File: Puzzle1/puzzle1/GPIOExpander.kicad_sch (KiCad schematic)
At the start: 4 parts, among them J2 Conn_01x16_Pin, U2 PCA9555D

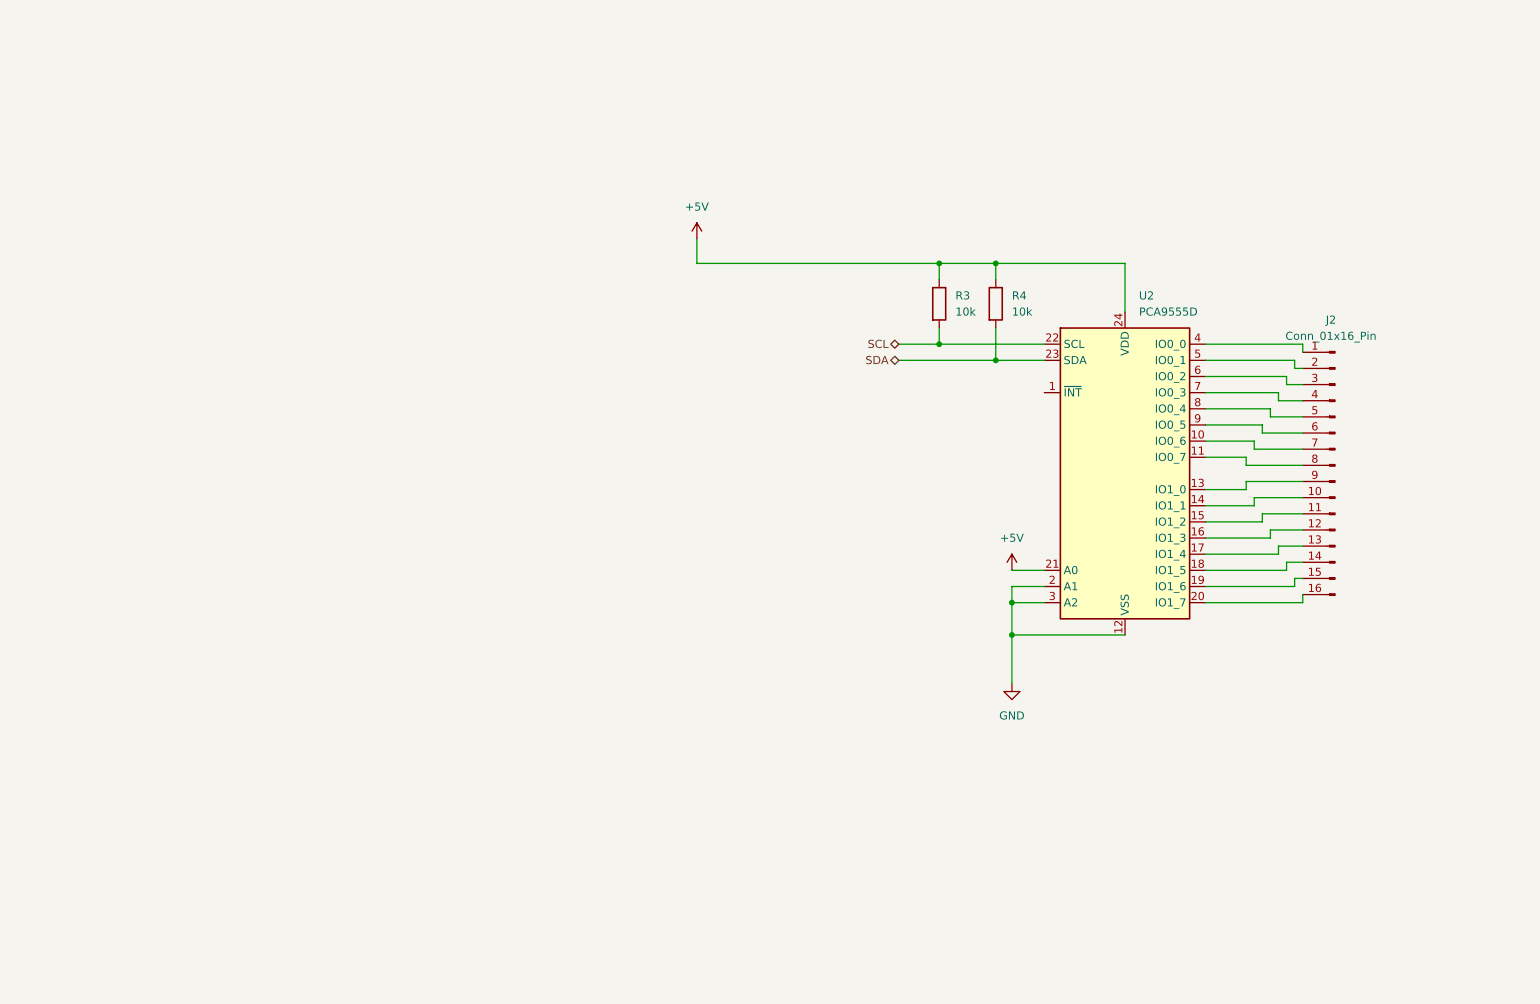
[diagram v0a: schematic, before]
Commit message: update
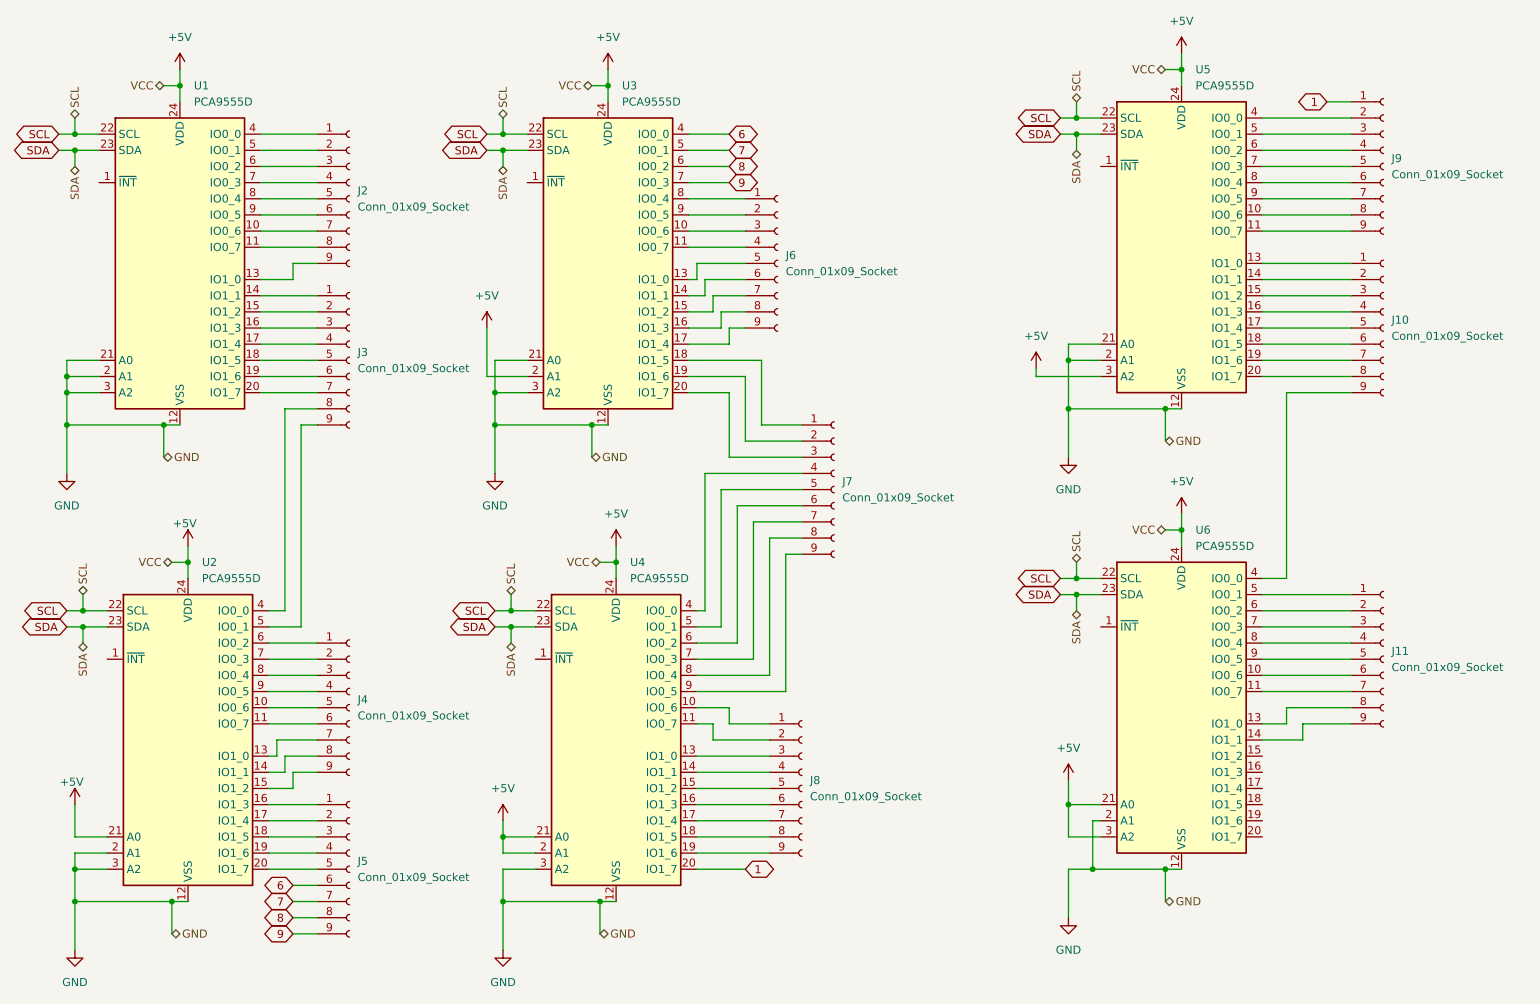
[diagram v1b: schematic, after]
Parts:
- removed J2: Conn_01x16_Pin, Connector_PinSocket_2.54mm:PinSocket_2x09_P2.54mm_Vertical, symbol Connector:Conn_01x16_Pin
- removed R3, R4: 10k, Resistor_SMD:R_0805_2012Metric, symbol Device:R
- added J10, J11, J2, J3, J4, J5, J6, J7, J8, J9: Conn_01x09_Socket, Connector_JST:JST_XH_B9B-XH-A_1x09_P2.50mm_Vertical, symbol Connector:Conn_01x09_Socket
- added U2, U3, U4, U5, U6: PCA9555D, Package_SO:SOIC-24W_7.5x15.4mm_P1.27mm, symbol Interface_Expansion:PCA9555D
- renumbered U2 to U1
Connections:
- net +5V: now also U2.21 (A0), U2.24 (VDD), U3.2 (A1), U3.24 (VDD), U4.2 (A1), U4.21 (A0), U4.24 (VDD), U5.24 (VDD), U5.3 (A2), U6.21 (A0), U6.24 (VDD), U6.3 (A2); no longer U1.21 (A0)
- net GND: now also U1.21 (A0), U2.12 (VSS), U2.2 (A1), U2.3 (A2), U3.12 (VSS), U3.21 (A0), U3.3 (A2), U4.12 (VSS), U4.3 (A2), U5.12 (VSS), U5.2 (A1), U5.21 (A0), U6.12 (VSS), U6.2 (A1)
- net SCL: now also U2.22 (SCL), U3.22 (SCL), U4.22 (SCL), U5.22 (SCL), U6.22 (SCL)
- net SDA: now also U2.23 (SDA), U3.23 (SDA), U4.23 (SDA), U5.23 (SDA), U6.23 (SDA)
- net at U1.4 (IO0_0): now also J2.1 (Pin_1)
- net at U1.14 (IO1_1): now also J3.1 (Pin_1)
- net at U1.15 (IO1_2): now also J3.2 (Pin_2)
- net at U1.16 (IO1_3): now also J3.3 (Pin_3)
- net at U1.17 (IO1_4): now also J3.4 (Pin_4)
- net at U1.18 (IO1_5): now also J3.5 (Pin_5)
- net at U1.19 (IO1_6): now also J3.6 (Pin_6)
- net at U1.20 (IO1_7): now also J3.7 (Pin_7)
- net at U1.5 (IO0_1): now also J2.2 (Pin_2)
- net at U1.6 (IO0_2): now also J2.3 (Pin_3)
- net at U1.7 (IO0_3): now also J2.4 (Pin_4)
- net at U1.8 (IO0_4): now also J2.5 (Pin_5)
- net at U1.9 (IO0_5): now also J2.6 (Pin_6)
- net at U1.10 (IO0_6): now also J2.7 (Pin_7)
- net at U1.11 (IO0_7): now also J2.8 (Pin_8)
- net at U1.13 (IO1_0): now also J2.9 (Pin_9)
- new net: J5.1 (Pin_1), U2.16 (IO1_3)
- new net: J5.2 (Pin_2), U2.17 (IO1_4)
- new net: J5.3 (Pin_3), U2.18 (IO1_5)
- new net: J5.4 (Pin_4), U2.19 (IO1_6)
- new net: J5.5 (Pin_5), U2.20 (IO1_7)
- new net: J10.1 (Pin_1), U5.13 (IO1_0)
- new net: J10.2 (Pin_2), U5.14 (IO1_1)
- new net: J10.3 (Pin_3), U5.15 (IO1_2)
- new net: J10.4 (Pin_4), U5.16 (IO1_3)
- new net: J10.5 (Pin_5), U5.17 (IO1_4)
- new net: J10.6 (Pin_6), U5.18 (IO1_5)
- new net: J10.7 (Pin_7), U5.19 (IO1_6)
- new net: J10.8 (Pin_8), U5.20 (IO1_7)
- new net: J10.9 (Pin_9), U6.4 (IO0_0)
- new net: J6.3 (Pin_3), U3.10 (IO0_6)
- new net: J6.4 (Pin_4), U3.11 (IO0_7)
- new net: J6.5 (Pin_5), U3.13 (IO1_0)
- new net: J6.6 (Pin_6), U3.14 (IO1_1)
- new net: J6.7 (Pin_7), U3.15 (IO1_2)
- new net: J6.8 (Pin_8), U3.16 (IO1_3)
- new net: J6.9 (Pin_9), U3.17 (IO1_4)
- new net: J7.1 (Pin_1), U3.18 (IO1_5)
- new net: J7.2 (Pin_2), U3.19 (IO1_6)
- new net: J7.3 (Pin_3), U3.20 (IO1_7)
- new net: J6.1 (Pin_1), U3.8 (IO0_4)
- new net: J6.2 (Pin_2), U3.9 (IO0_5)
- new net: J11.1 (Pin_1), U6.5 (IO0_1)
- new net: J11.2 (Pin_2), U6.6 (IO0_2)
- new net: J11.3 (Pin_3), U6.7 (IO0_3)
- new net: J11.4 (Pin_4), U6.8 (IO0_4)
- new net: J11.5 (Pin_5), U6.9 (IO0_5)
- new net: J11.6 (Pin_6), U6.10 (IO0_6)
- new net: J11.7 (Pin_7), U6.11 (IO0_7)
- new net: J11.8 (Pin_8), U6.13 (IO1_0)
- new net: J11.9 (Pin_9), U6.14 (IO1_1)
- new net: J8.1 (Pin_1), U4.10 (IO0_6)
- new net: J8.2 (Pin_2), U4.11 (IO0_7)
- new net: J8.3 (Pin_3), U4.13 (IO1_0)
- new net: J8.4 (Pin_4), U4.14 (IO1_1)
- new net: J8.5 (Pin_5), U4.15 (IO1_2)
- new net: J8.6 (Pin_6), U4.16 (IO1_3)
- new net: J8.7 (Pin_7), U4.17 (IO1_4)
- new net: J8.8 (Pin_8), U4.18 (IO1_5)
- new net: J8.9 (Pin_9), U4.19 (IO1_6)
- new net: J9.8 (Pin_8), U5.10 (IO0_6)
- new net: J9.9 (Pin_9), U5.11 (IO0_7)
- new net: J9.2 (Pin_2), U5.4 (IO0_0)
- new net: J9.3 (Pin_3), U5.5 (IO0_1)
- new net: J9.4 (Pin_4), U5.6 (IO0_2)
- new net: J9.5 (Pin_5), U5.7 (IO0_3)
- new net: J9.6 (Pin_6), U5.8 (IO0_4)
- new net: J9.7 (Pin_7), U5.9 (IO0_5)
- new net: J4.1 (Pin_1), U2.6 (IO0_2)
- new net: J4.2 (Pin_2), U2.7 (IO0_3)
- new net: J4.3 (Pin_3), U2.8 (IO0_4)
- new net: J4.4 (Pin_4), U2.9 (IO0_5)
- new net: J4.5 (Pin_5), U2.10 (IO0_6)
- new net: J4.6 (Pin_6), U2.11 (IO0_7)
- new net: J4.7 (Pin_7), U2.13 (IO1_0)
- new net: J4.8 (Pin_8), U2.14 (IO1_1)
- new net: J4.9 (Pin_9), U2.15 (IO1_2)
- new net: J7.4 (Pin_4), U4.4 (IO0_0)
- new net: J7.5 (Pin_5), U4.5 (IO0_1)
- new net: J7.6 (Pin_6), U4.6 (IO0_2)
- new net: J7.7 (Pin_7), U4.7 (IO0_3)
- new net: J7.8 (Pin_8), U4.8 (IO0_4)
- new net: J7.9 (Pin_9), U4.9 (IO0_5)
- new net: J3.8 (Pin_8), U2.4 (IO0_0)
- new net: J3.9 (Pin_9), U2.5 (IO0_1)
- new net 1: J9.1 (Pin_1), U4.20 (IO1_7)
- new net 6: J5.6 (Pin_6), U3.4 (IO0_0)
- new net 7: J5.7 (Pin_7), U3.5 (IO0_1)
- new net 8: J5.8 (Pin_8), U3.6 (IO0_2)
- new net 9: J5.9 (Pin_9), U3.7 (IO0_3)
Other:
- moved on the sheet: U1

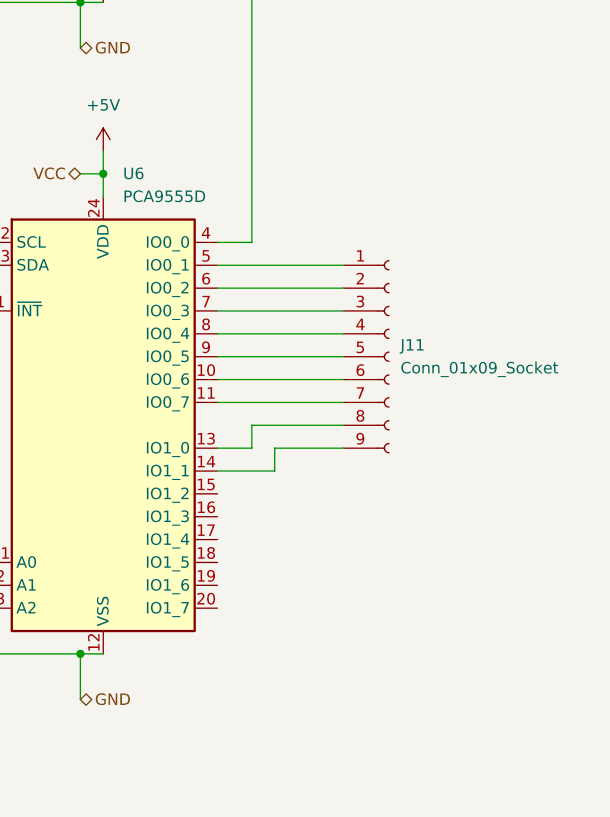
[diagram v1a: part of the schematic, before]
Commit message: update
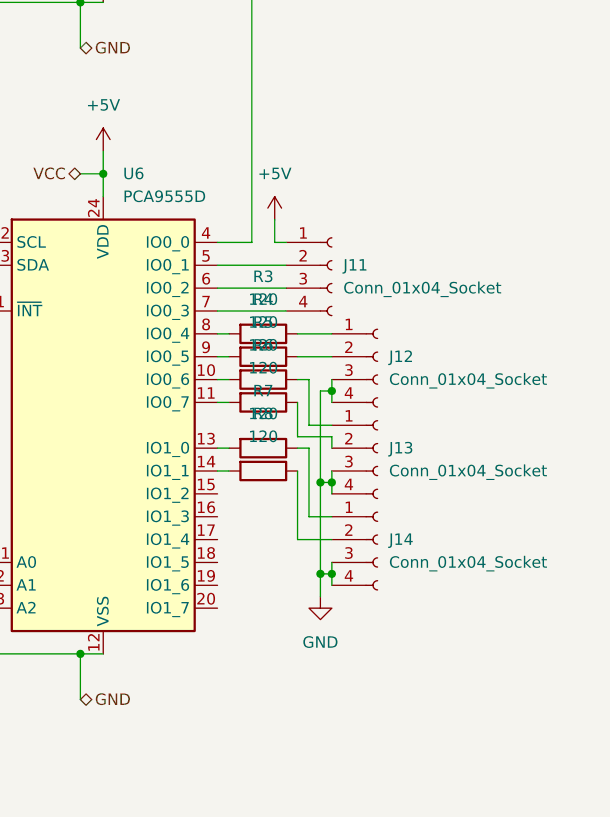
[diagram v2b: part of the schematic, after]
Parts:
- removed J11: Conn_01x09_Socket, Connector_JST:JST_XH_B9B-XH-A_1x09_P2.50mm_Vertical, symbol Connector:Conn_01x09_Socket
- added J11, J12, J13, J14: Conn_01x04_Socket, Connector_JST:JST_XH_B4B-XH-A_1x04_P2.50mm_Vertical, symbol Connector:Conn_01x04_Socket
- added R3, R4, R5, R6, R7, R8: 120, Resistor_SMD:R_0603_1608Metric, symbol Device:R
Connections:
- net +5V: now also J11.1 (Pin_1)
- net GND: now also J12.3 (Pin_3), J12.4 (Pin_4), J13.3 (Pin_3), J13.4 (Pin_4), J14.3 (Pin_3), J14.4 (Pin_4)
- net at U6.5 (IO0_1): now also J11.2 (Pin_2)
- net at U6.6 (IO0_2): now also J11.3 (Pin_3)
- net at U6.7 (IO0_3): now also J11.4 (Pin_4)
- net at U6.8 (IO0_4): now also R3.2
- net at U6.9 (IO0_5): now also R4.2
- net at U6.10 (IO0_6): now also R5.2
- net at U6.11 (IO0_7): now also R6.2
- net at U6.13 (IO1_0): now also R7.2
- net at U6.14 (IO1_1): now also R8.2
- new net: J12.2 (Pin_2), R4.1
- new net: J14.2 (Pin_2), R8.1
- new net: J12.1 (Pin_1), R3.1
- new net: J14.1 (Pin_1), R7.1
- new net: J13.1 (Pin_1), R5.1
- new net: J13.2 (Pin_2), R6.1
